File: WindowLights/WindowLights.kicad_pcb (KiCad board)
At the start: 2 copper layers, 40.6 x 101.6 mm, 9 parts, among them J101 IN, J102 OUT, U101 WS2811

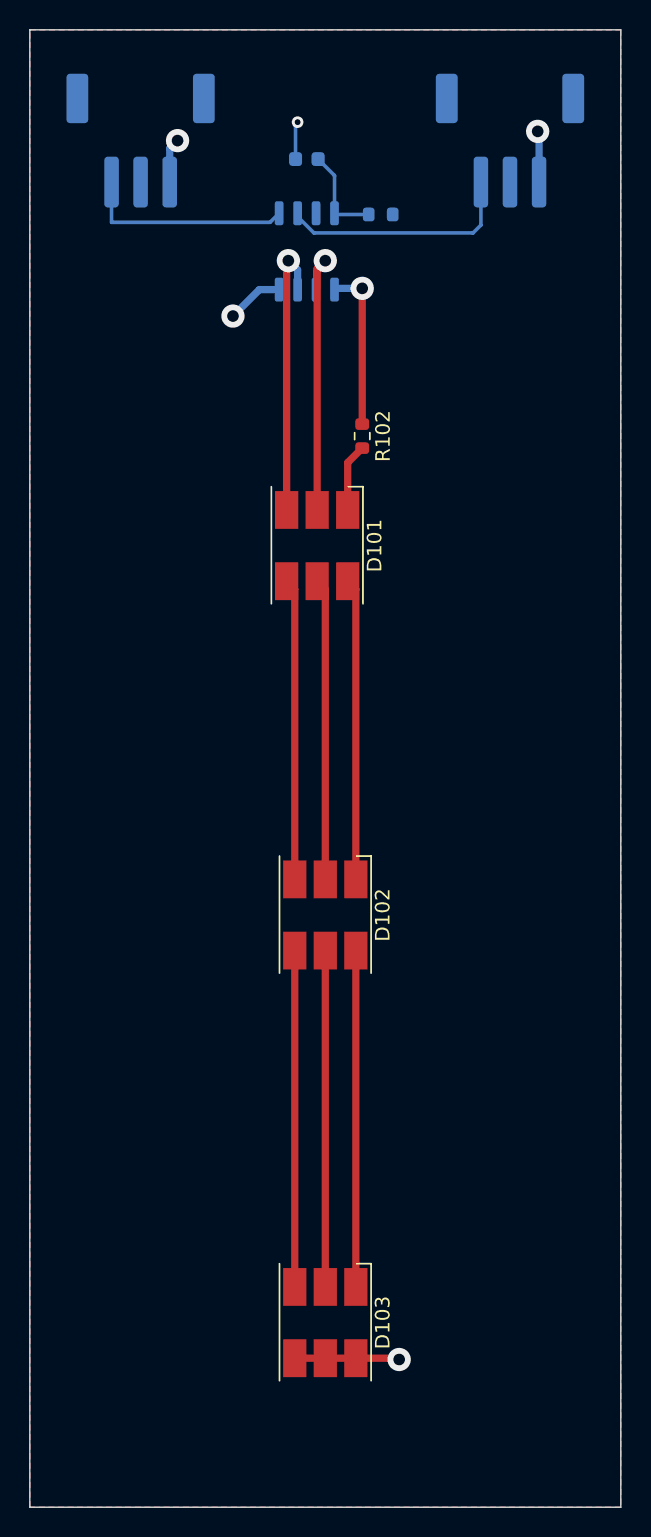
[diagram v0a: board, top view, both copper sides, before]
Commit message: Update for new window sizes.
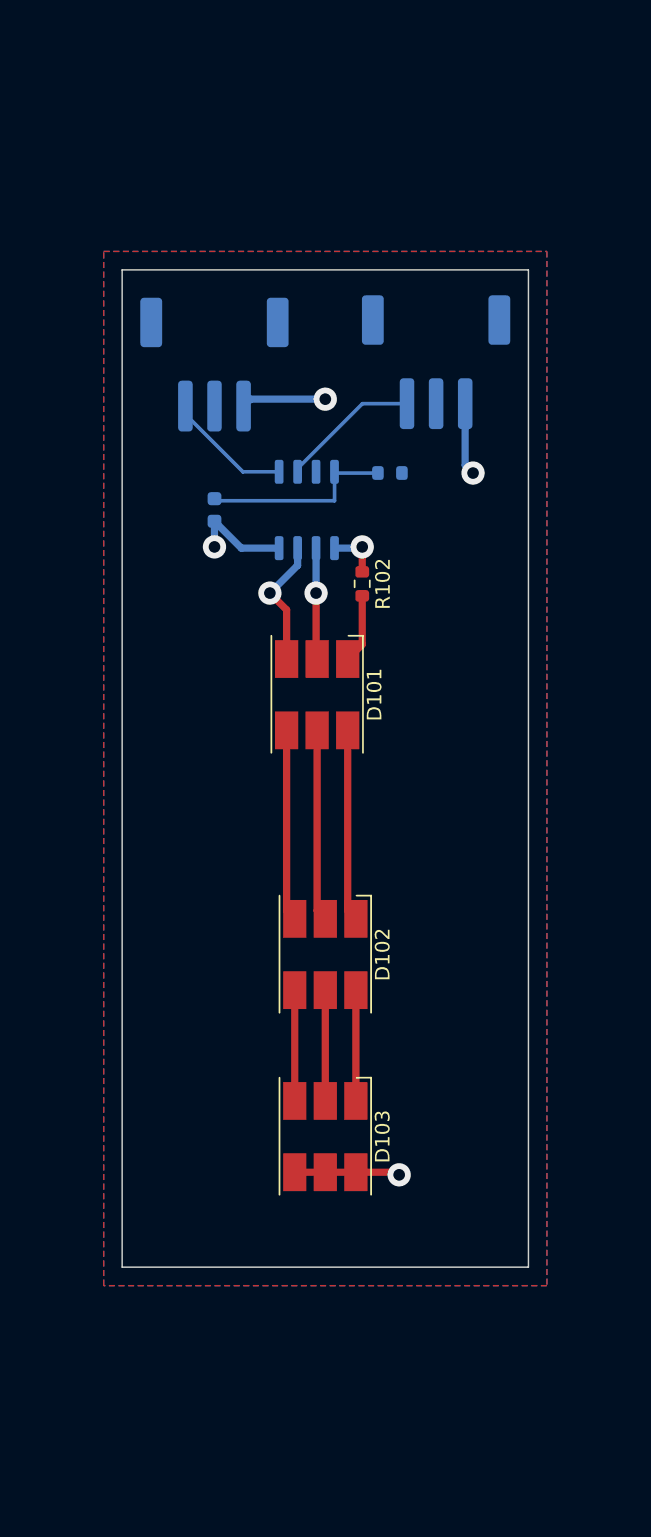
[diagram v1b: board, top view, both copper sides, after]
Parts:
- moved C101 25.0 mm to (116.8, 71.1), turned to 90 degrees
- moved R101 17.8 mm to (128.9, 68.6)
- moved U101 17.8 mm to (123.2, 71.1)
- moved J102 16.2 mm to (116.8, 61.1)
- moved J101 16.1 mm to (132.1, 61.0)
- moved D103 12.8 mm to (124.5, 114.2)
- moved D101 10.2 mm to (123.9, 83.8)
- moved R102 10.2 mm to (127.0, 76.2)
- moved D102 2.72 mm to (124.5, 101.7)
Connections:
- D101 pad 3: Net-(D101-Pad2) -> Net-(D101-Pad3)
- U101 pad 3: Net-(D101-Pad2) -> Net-(D101-Pad3)
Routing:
- net Net-(D101-Pad2): track 39.1 -> 7.66 mm, vias 2 -> 1
- net Net-(D102-Pad6): track 23.1 -> 7.62 mm
- net Net-(D102-Pad5): track 23.1 -> 7.62 mm
- net Net-(D102-Pad4): track 23.1 -> 7.62 mm
- net Net-(D101-Pad3): track 0.00 -> 8.89 mm, vias 0 -> 1
- net Net-(R102-Pad1): track 11.3 -> 3.66 mm
- net Net-(D101-Pad6): track 20.7 -> 13.2 mm
- net Net-(D101-Pad4): track 20.7 -> 13.2 mm
- net Net-(D101-Pad5): track 20.7 -> 13.2 mm
- net Net-(J101-Pad1): track 16.5 -> 9.60 mm
- net Net-(C101-Pad2): track 6.58 -> 13.3 mm
- net Net-(J102-Pad1): track 14.6 -> 8.65 mm
- net GND: track 13.1 -> 17.9 mm, vias 4 -> 3
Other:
- board size 40.6 x 101.6 mm -> 27.9 x 68.6 mm
